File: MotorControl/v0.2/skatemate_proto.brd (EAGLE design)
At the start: 126.5 x 87.3 mm, 104 parts, among them IC1 REG1117, Q1 IRF740, Q2 IRF740, Q3 IRF740, Q4 IRF740, Q5 IRF740, Q6 IRF740, U1 DRV8301DCAR

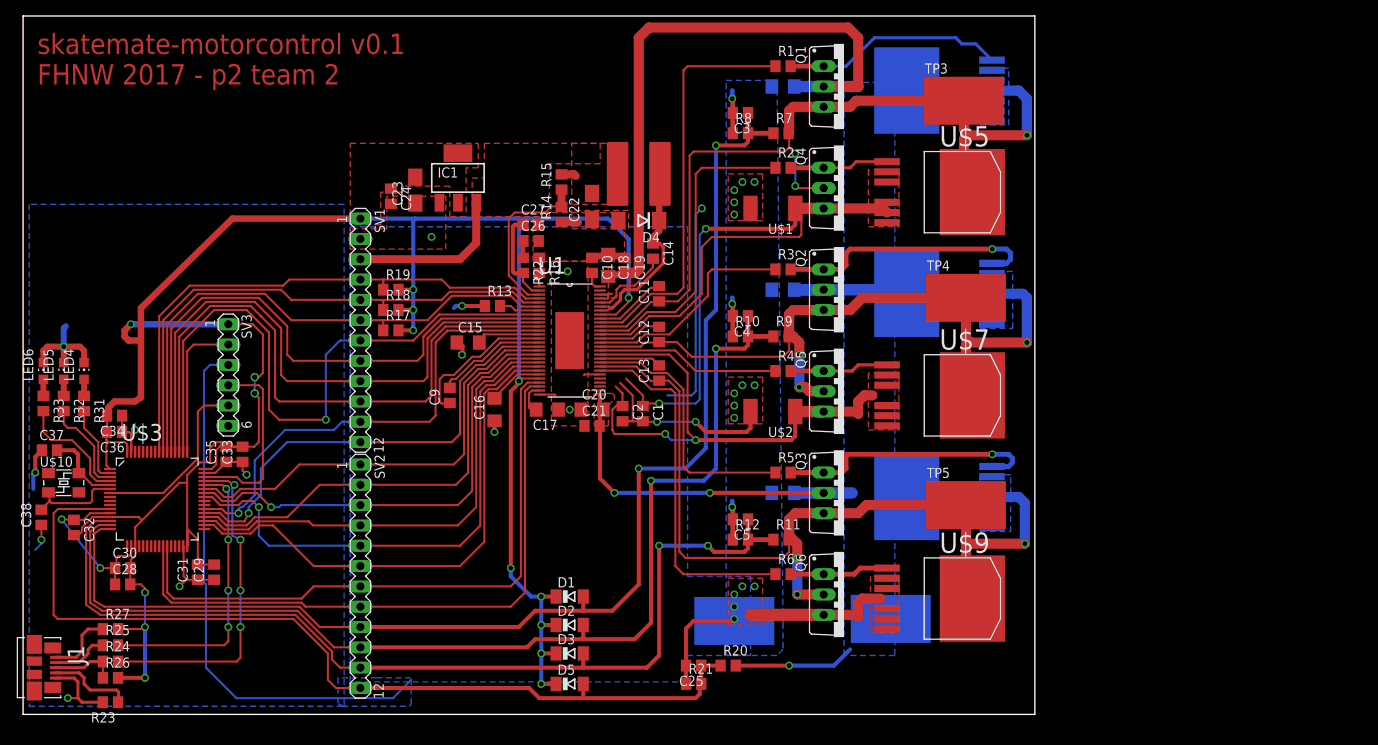
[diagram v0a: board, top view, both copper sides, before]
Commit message: layouting on v0.2
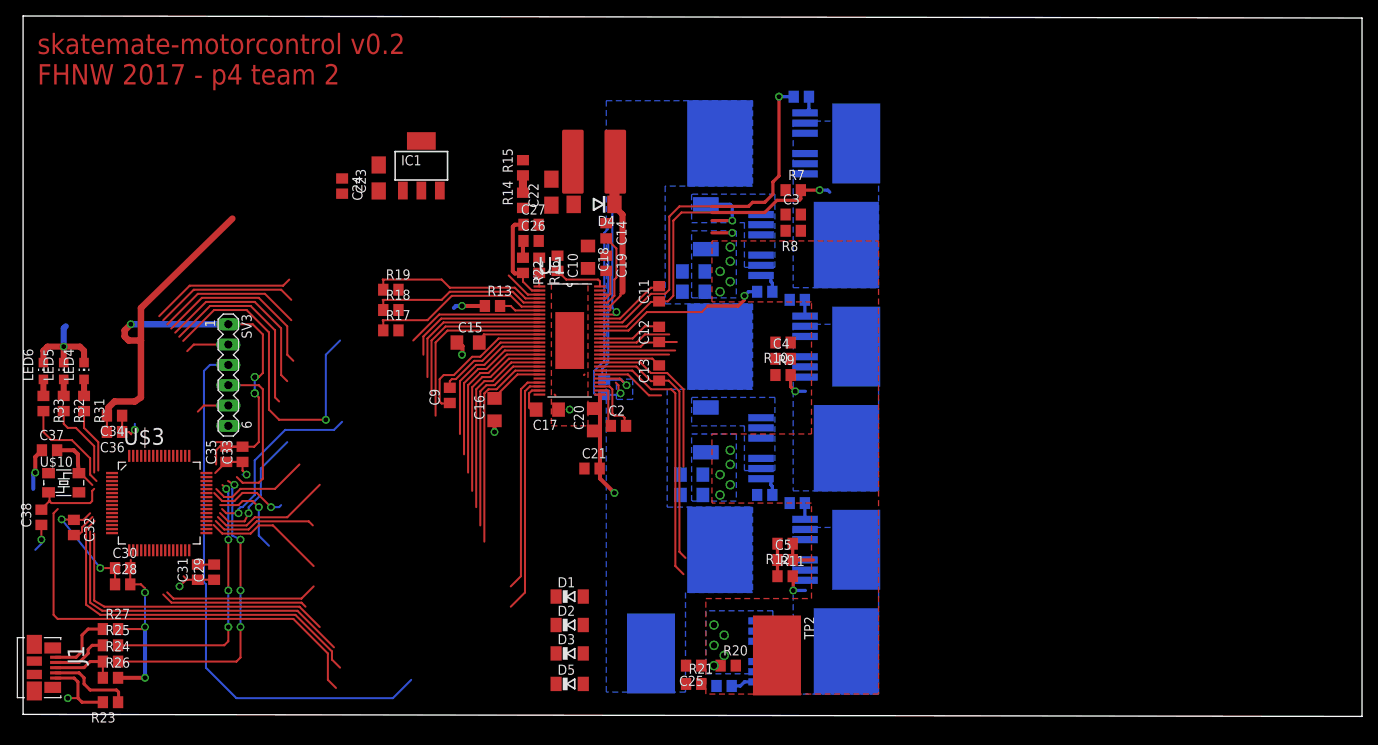
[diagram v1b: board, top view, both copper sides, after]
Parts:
- removed Q1, Q2, Q3, Q4, Q5, Q6: IRF740, transistor-power:TO220BV
- removed SV1, SV2: (no value), skatemate:MA12-1
- added C39: 2u2, skatemate:C1206
- TP1: value TPSMD_M_1006 -> SUPPLY
- TP2: value TPSMD_M_1006 -> GND
- TP3: value TPSMD_M_1006 -> PH_A
- TP4: value TPSMD_M_1006 -> PH_B
- TP5: value TPSMD_M_1006 -> PH_C
- moved TP1 30.3 mm to (78.5, 7.62), turned to 90 degrees
- moved C6 28.0 mm to (83.8, 52.8), turned to 180 degrees
- moved C7 25.8 mm to (83.6, 30.0), turned to 180 degrees
- moved U$4 24.3 mm to (91.2, 71.4)
- moved U$6 24.3 mm to (91.2, 46.0)
- moved U$8 24.3 mm to (91.2, 20.6)
- moved U$5 17.1 mm to (98.8, 58.7), flipped to the bottom, turned to 90 degrees
- moved U$7 17.1 mm to (98.8, 33.3), flipped to the bottom, turned to 90 degrees
- moved U$9 17.1 mm to (98.8, 7.87), flipped to the bottom, turned to 90 degrees
- moved R6 15.8 mm to (87.6, 3.56), flipped to the bottom, turned to 180 degrees
- moved R4 15.7 mm to (92.7, 27.4), flipped to the bottom, turned to 180 degrees
- moved R2 15.7 mm to (92.7, 52.8), flipped to the bottom, turned to 180 degrees
- moved TP4 15.0 mm to (104.1, 46.0), flipped to the bottom, turned to 270 degrees
- moved TP5 14.8 mm to (104.1, 20.6), flipped to the bottom, turned to 270 degrees
- moved TP3 14.5 mm to (104.1, 71.4), flipped to the bottom, turned to 270 degrees
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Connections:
- net +5V: no longer SV1.3
- net ASENSE: no longer SV2.9
- net BSENSE: no longer SV2.10
- net CSENSE: no longer SV2.11
- net DRV_DCCAL: no longer SV1.11
- net DRV_EN_GATE: no longer SV1.12
- net DRV_NCS: no longer SV1.7
- net DRV_NFAULT: no longer SV1.6
- net DRV_NOCTW: no longer SV1.5
- net DRV_PWRGD: no longer SV1.4
- net DRV_SCK: no longer SV1.10
- net DRV_SDI: no longer SV1.8
- net DRV_SDO: no longer SV1.9
- net DRV_SOA: no longer SV2.7
- net DRV_SOB: no longer SV2.8
- net GND: now also C39.2; no longer Q6.S, SV1.2
- net INH_A: no longer SV2.1
- net INH_B: no longer SV2.3
- net INH_C: no longer SV2.5
- net INL_A: no longer SV2.2
- net INL_B: no longer SV2.4
- net INL_C: no longer SV2.6
- net N$10: no longer Q2.G
- net N$11: no longer Q3.G
- net N$12: no longer Q6.G
- net N$7: no longer Q1.G
- net N$8: no longer Q4.G
- net N$9: no longer Q5.G
- net PH_A: no longer Q1.S, Q4.D
- net PH_B: no longer Q2.S, Q5.D
- net PH_C: no longer Q3.S, Q6.D
- net SN_A: no longer Q4.S
- net SN_B: no longer Q5.S
- net SSENSE: no longer SV2.12
- net SUPPLY: now also C39.1; no longer Q1.D, Q2.D, Q3.D
- net VCC: no longer SV1.1
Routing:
- net VCC: track 317.3 -> 125.5 mm, vias 16 -> 7
- net SUPPLY: track 162.9 -> 18.9 mm, vias 3 -> 1
- net ASENSE: track 157.2 -> 37.8 mm, vias 2 -> 0
- net BSENSE: track 139.6 -> 41.6 mm, vias 2 -> 0
- net PH_B: track 93.3 -> 13.4 mm, vias 3 -> 1
- net PH_C: track 113.0 -> 35.8 mm, vias 3 -> 1
- net GND: track 267.1 -> 193.5 mm, vias 36 -> 30
- net CSENSE: track 122.8 -> 50.4 mm, vias 2 -> 0
- net PH_A: track 107.5 -> 42.0 mm, vias 3 -> 1
- net SN_A: track 95.8 -> 34.1 mm
- net SSENSE: track 115.1 -> 54.5 mm
- net SN_B: track 65.9 -> 14.2 mm, vias 2 -> 0
- net DRV_SCK: track 78.8 -> 45.0 mm
- net DRV_SDO: track 75.4 -> 42.8 mm
- net DRV_SDI: track 71.9 -> 39.9 mm
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- added copper zone on layer 16, net SN_A
- added copper zone on layer 16, net SN_B
- removed copper zone on layer 1, net +5V
- removed copper zone on layer 1, net SN_A
- removed copper zone on layer 1, net SN_B
- removed copper zone on layer 1, net SUPPLY
- removed copper zone on layer 1, net VCC
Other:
- board size 126.5 x 87.3 mm -> 167.4 x 87.6 mm
- board text added: "FHNW 2017 - p4 team 2"
- board text added: "skatemate-motorcontrol v0.2"
- board text removed: "FHNW 2017 - p2 team 2"
- board text removed: "skatemate-motorcontrol v0.1"
